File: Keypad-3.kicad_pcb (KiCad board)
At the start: 2 copper layers, 69.1 x 49 mm, 23 parts, among them J1 USB_C_Receptacle_USB2.0, SW1 SW_Push, U1 ATmega32U4-A, U2 SRV05-4, Y1 16MHz

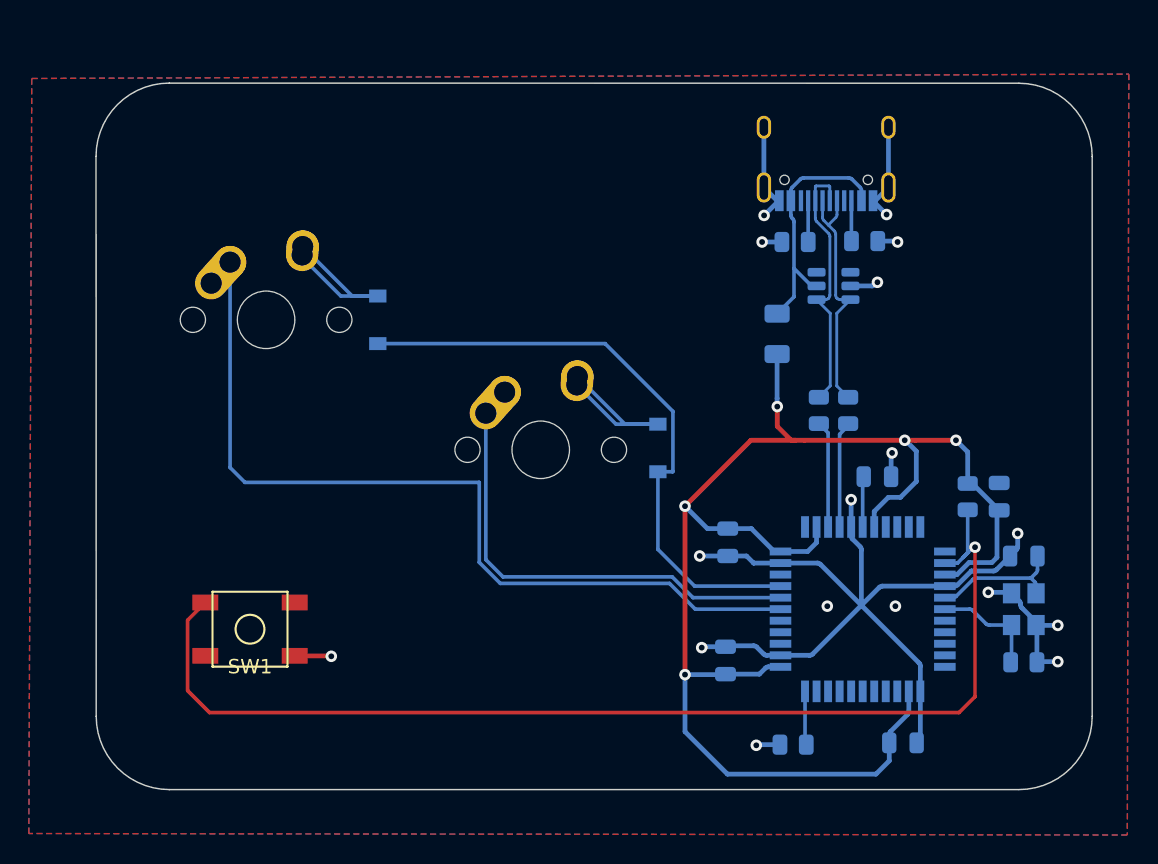
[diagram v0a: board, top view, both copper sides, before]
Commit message: Made the gerber files
:D
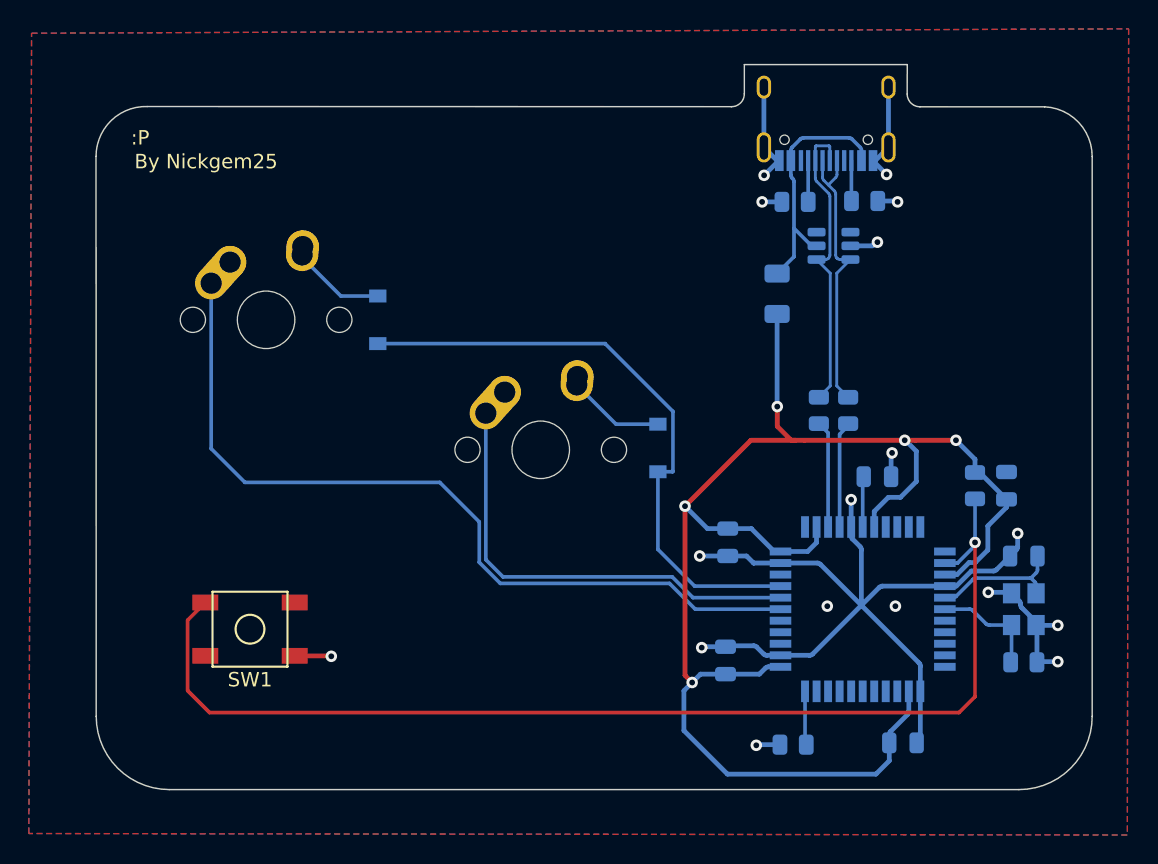
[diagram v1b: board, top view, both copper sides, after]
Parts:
- moved F1 2.78 mm to (194.0, 109.9)
- moved J1 2.78 mm to (197.4, 96.6)
- moved R5 2.78 mm to (200.1, 103.4)
- moved R6 2.78 mm to (195.3, 103.5)
- moved U2 2.78 mm to (198.0, 106.6)
- moved C4 0.92 mm to (210.0, 123.2)
- moved R1 0.92 mm to (207.8, 123.2)
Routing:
- net Net-(D2-Pad2): track 13.7 -> 6.76 mm
- net Net-(D1-Pad2): track 13.2 -> 6.52 mm
- net D+: track 17.5 -> 20.3 mm
- net D-: track 18.5 -> 21.3 mm
- net +5V: track 104.6 -> 107.3 mm
- net COL0: track 59.7 -> 57.2 mm
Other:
- board size 69.1 x 49 mm -> 69.1 x 50.3 mm
- board text added: ":P"
- board text added: "By Nickgem25"
